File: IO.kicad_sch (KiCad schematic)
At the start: 154 parts, among them J1 RJ45_Bel_SI-60062-F, J11 Screw_Terminal_01x06, J12 Screw_Terminal_01x03, J13 Screw_Terminal_01x02, J14 Screw_Terminal_01x02, J15 Screw_Terminal_01x02, J16 Screw_Terminal_01x02, J4 Conn_01x06, J9 Screw_Terminal_01x06, K1 Relay_SPDT, K2 Relay_SPDT, K3 Relay_SPDT, K4 Relay_SPDT, Q5 NMOS, Q6 NMOS, Q7 NMOS, Q8 NMOS, U4 W5500, U5 SFH617A-1X007T, U6 MAX485E, U7 SFH617A-1X007T, U8 SFH617A-1X007T, U9 SFH617A-1X007T, Y1 25MHz

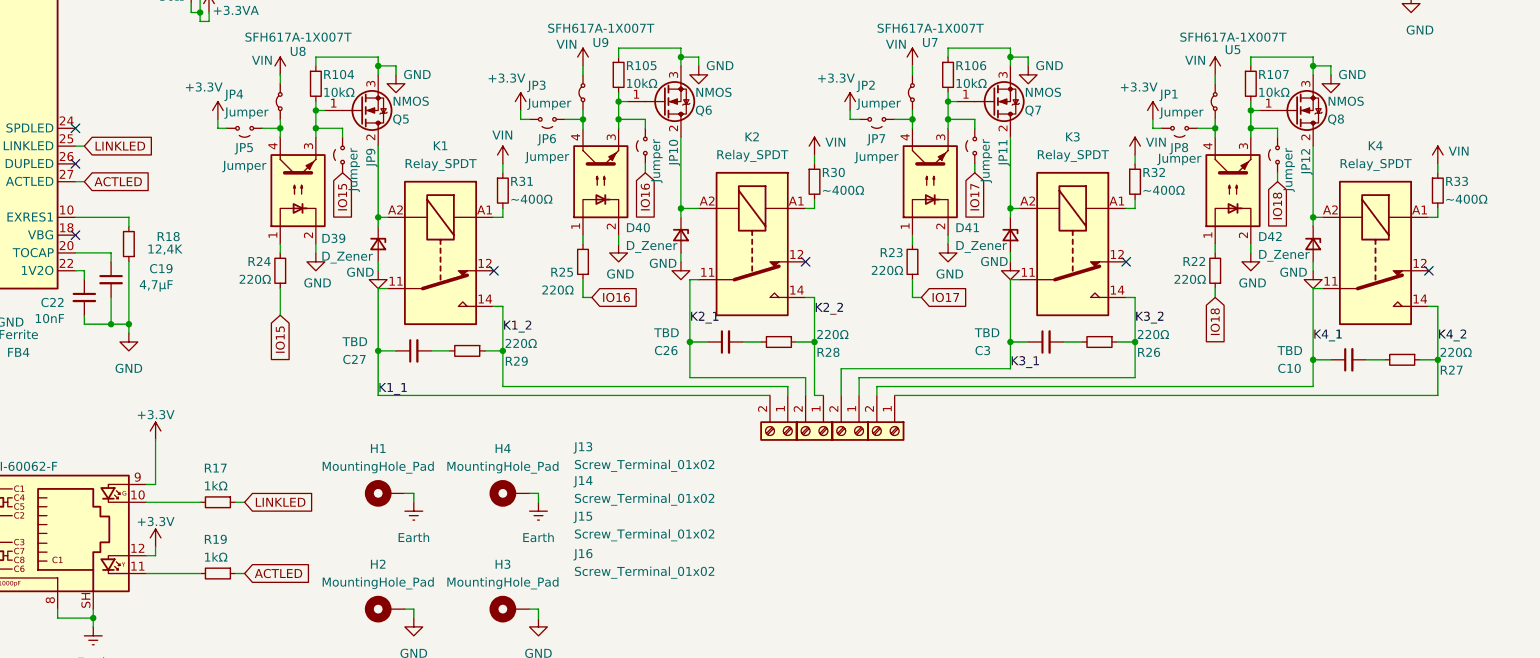
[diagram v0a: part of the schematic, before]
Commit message: development
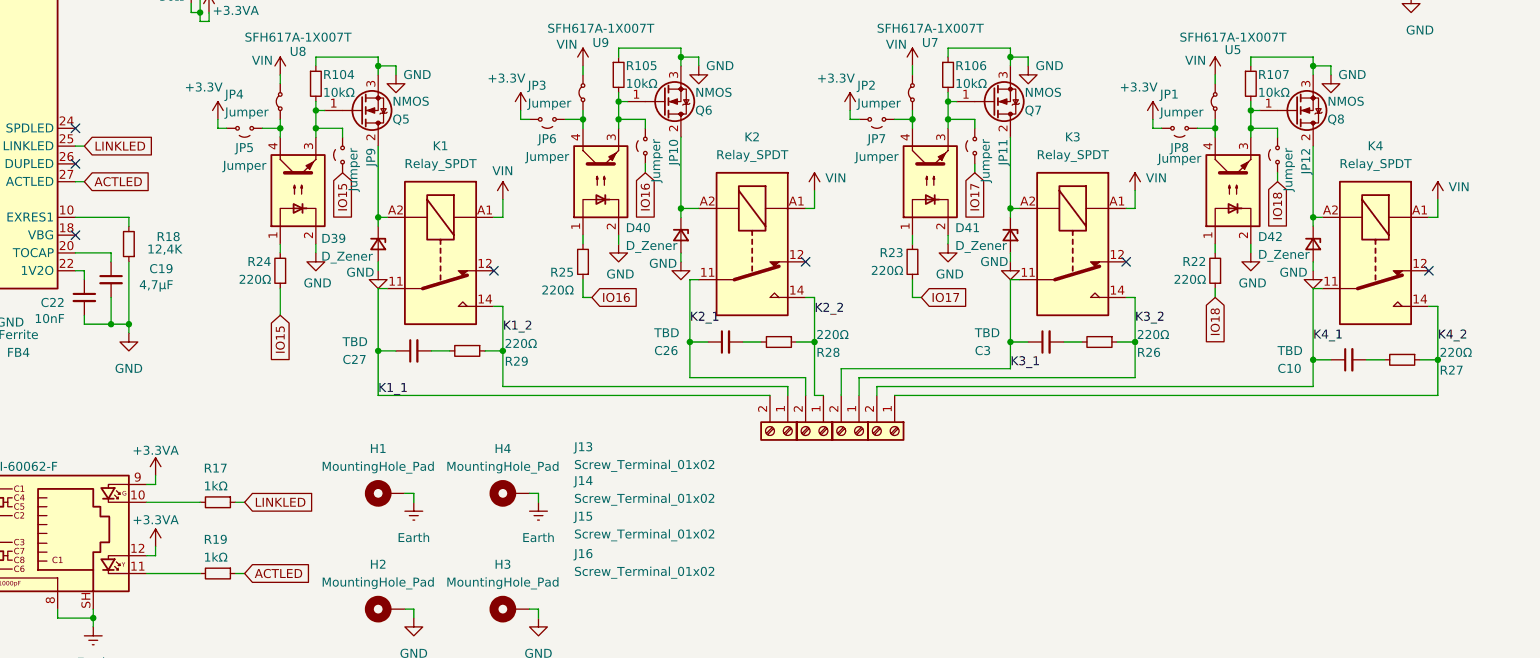
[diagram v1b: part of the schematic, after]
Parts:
- removed R30, R31, R32, R33: ~400Ω, Resistor_SMD:R_1206_3216Metric, symbol Device:R_Small
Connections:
- net +3.3V: no longer J1.12, J1.9
- net +3.3VA: now also J1.12, J1.9
- net VIN: now also K1.A1, K2.A1, K3.A1, K4.A1
